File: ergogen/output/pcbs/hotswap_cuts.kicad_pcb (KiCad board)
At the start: 2 copper layers, 220.4 x 89.6 mm, 37 parts

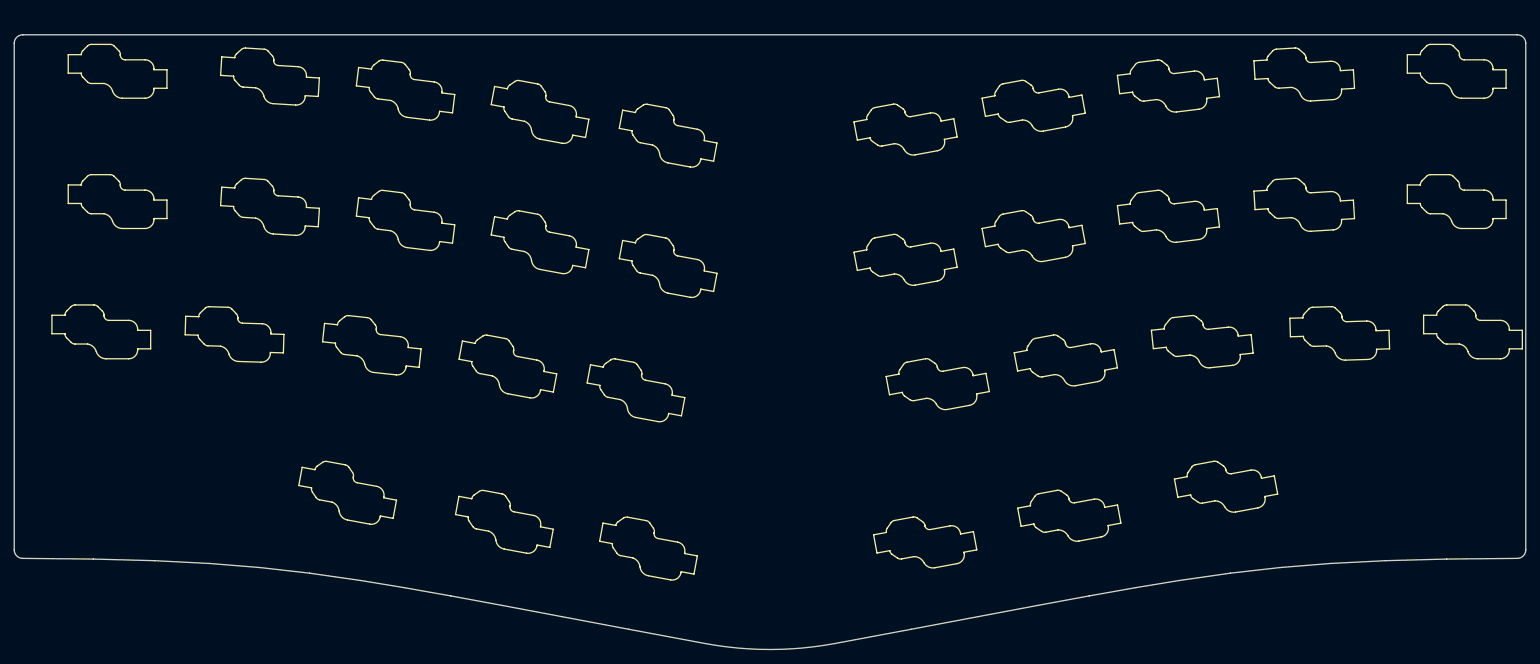
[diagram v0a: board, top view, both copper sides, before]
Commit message: release
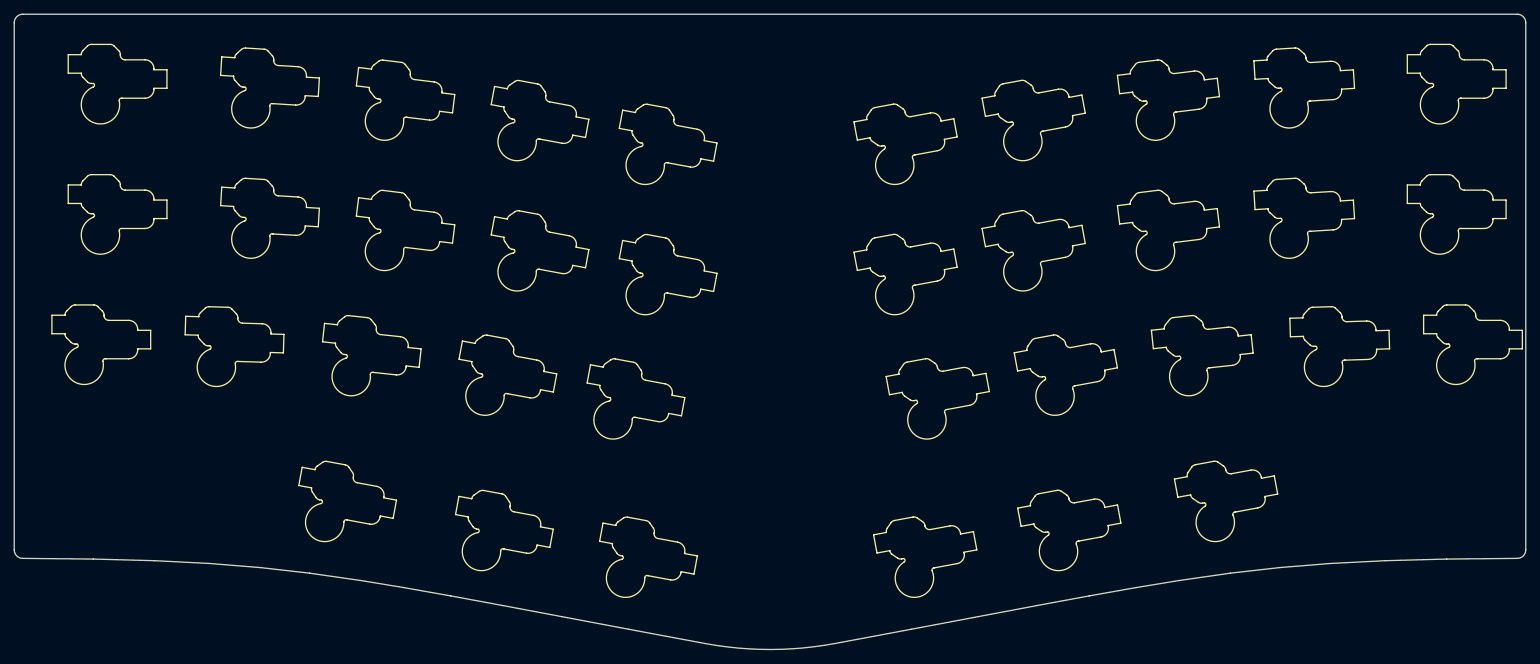
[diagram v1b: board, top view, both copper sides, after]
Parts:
- GL1, GL10, GL11, GL12, GL13, GL14, GL15, GL16, GL17, GL18, GL19, GL2, GL20, GL21, GL22, GL23, GL24, GL25, GL26, GL27, GL28, GL29, GL3, GL30, GL31, GL32, GL33, GL34, GL35, GL36, GL4, GL5, GL6, GL7, GL8, GL9: footprint hotswap_cutout -> hotswap_v2_pin_cutout
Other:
- board size 220.4 x 89.6 mm -> 220.4 x 92.6 mm
